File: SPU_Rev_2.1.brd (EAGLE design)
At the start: 127.6 x 101.6 mm, 255 parts, among them Q1 12MHz

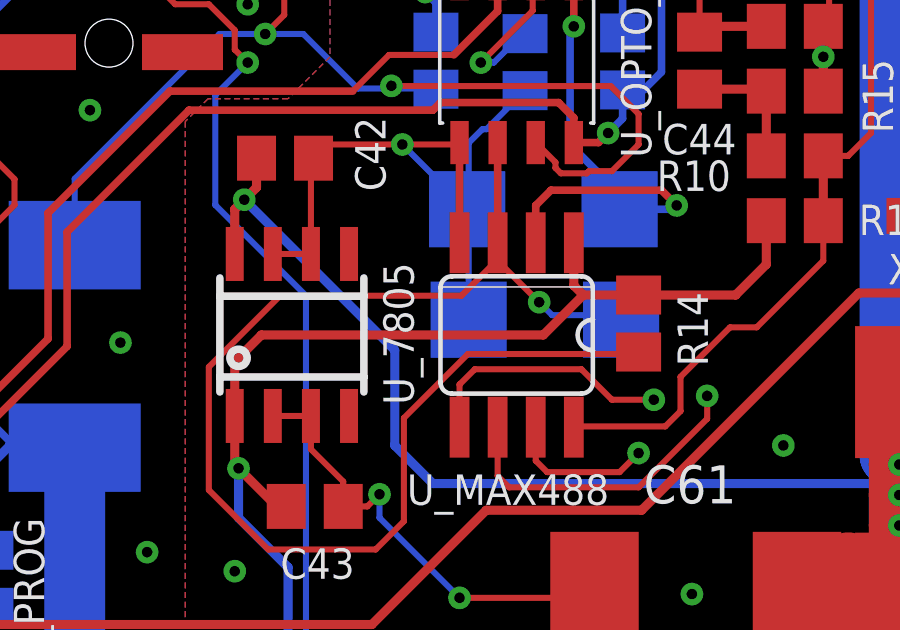
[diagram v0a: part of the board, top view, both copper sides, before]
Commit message: foo
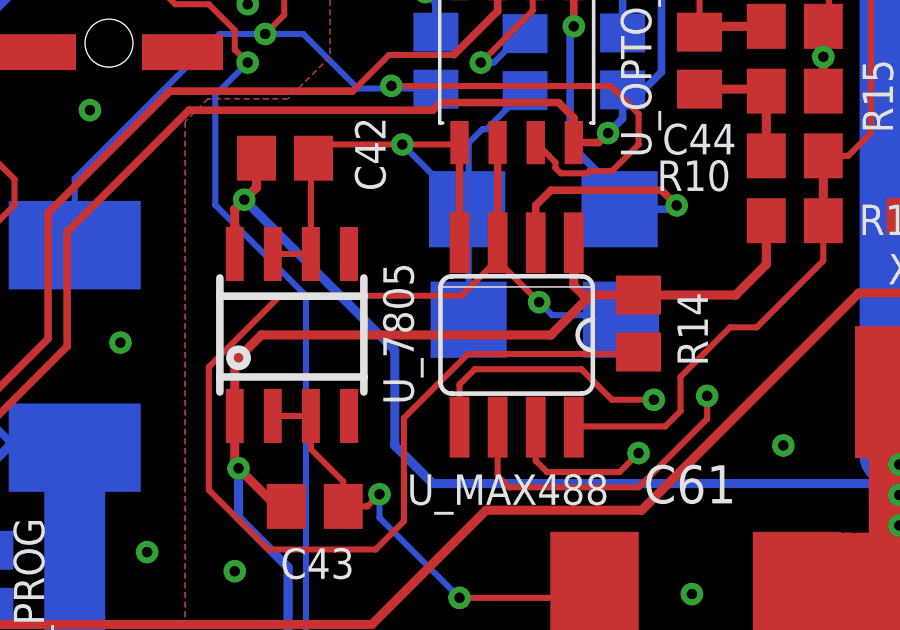
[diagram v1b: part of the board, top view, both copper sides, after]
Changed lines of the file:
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@@
 <drawing>
 <settings>
-<setting alwaysvectorfont="no"/>
+<setting alwaysvectorfont="yes"/>
 <setting verticaltext="up"/>
 </settings>
@@
 <wire x1="15.416" y1="30.783" x2="15.416" y2="31.261" width="0.2032" layer="16"/>
 <wire x1="16.454" y1="34.361" x2="15.367" y2="33.274" width="0.2032" layer="16"/>
-<wire x1="99.568" y1="91.948" x2="101.092" y2="95.123" width="0" layer="19" extent="16-16"/>
-<wire x1="64.4398" y1="61.5696" x2="62.484" y2="61.595" width="0" layer="19" extent="16-16"/>
-<wire x1="40.767" y1="11.176" x2="41.187" y2="9.271" width="0" layer="19" extent="1-1"/>
-<wire x1="71.628" y1="65.532" x2="73.66" y2="66.04" width="0" layer="19" extent="1-1"/>
-<wire x1="12.446" y1="77.597" x2="14.351" y2="78.486" width="0" layer="19" extent="1-1"/>
-<wire x1="38.608" y1="11.176" x2="40.767" y2="11.176" width="0" layer="19" extent="1-1"/>
-<wire x1="91.948" y1="63.881" x2="89.662" y2="63.119" width="0" layer="19" extent="1-1"/>
-<wire x1="90.805" y1="65.532" x2="91.948" y2="63.881" width="0" layer="19" extent="1-1"/>
-<wire x1="91.694" y1="73.787" x2="92.964" y2="71.628" width="0" layer="19" extent="16-16"/>
-<wire x1="97.409" y1="75.565" x2="99.06" y2="77.978" width="0" layer="19" extent="1-1"/>
-<wire x1="86.106" y1="9.525" x2="87.757" y2="7.112" width="0" layer="19" extent="1-1"/>
-<wire x1="67.31" y1="93.98" x2="64.262" y2="94.0054" width="0" layer="19" extent="1-1"/>
-<wire x1="38.735" y1="28.067" x2="39.37" y2="25.019" width="0" layer="19" extent="1-1"/>
-<wire x1="101.346" y1="82.931" x2="99.568" y2="85.598" width="0" layer="19" extent="16-16"/>
-<wire x1="91.694" y1="36.195" x2="91.313" y2="32.893" width="0" layer="19" extent="1-1"/>
-<wire x1="63.881" y1="72.39" x2="62.484" y2="69.215" width="0" layer="19" extent="16-16"/>
-<wire x1="91.186" y1="50.038" x2="89.662" y2="53.286" width="0" layer="19" extent="16-16"/>
-<wire x1="82.169" y1="94.742" x2="78.613" y2="93.8784" width="0" layer="19" extent="1-1"/>
-<wire x1="12.827" y1="26.543" x2="14.732" y2="23.239" width="0" layer="19" extent="1-1"/>
-<wire x1="12.827" y1="6.985" x2="13.208" y2="10.795" width="0" layer="19" extent="1-1"/>
-<wire x1="12.192" y1="84.328" x2="16.013" y2="83.6962" width="0" layer="19" extent="1-1"/>
-<wire x1="32.766" y1="45.212" x2="33.782" y2="49.024" width="0" layer="19" extent="1-1"/>
-<wire x1="26.797" y1="51.562" x2="22.733" y2="51.855" width="0" layer="19" extent="1-1"/>
-<wire x1="59.309" y1="32.512" x2="62.611" y2="30.045" width="0" layer="19" extent="16-16"/>
-<wire x1="102.87" y1="74.168" x2="99.568" y2="71.628" width="0" layer="19" extent="16-16"/>
-<wire x1="105.156" y1="71.755" x2="102.87" y2="74.168" width="0" layer="19" extent="1-1"/>
-<wire x1="103.632" y1="69.088" x2="105.156" y2="71.755" width="0" layer="19" extent="1-1"/>
-<wire x1="25.781" y1="45.339" x2="21.678" y2="46.101" width="0" layer="19" extent="16-16"/>
-<wire x1="40.64" y1="45.339" x2="38.7096" y2="49.149" width="0" layer="19" extent="1-1"/>
-<wire x1="17.272" y1="45.466" x2="19.812" y2="49.024" width="0" layer="19" extent="1-1"/>
-<wire x1="14.516" y1="44.461" x2="17.272" y2="45.466" width="0" layer="19" extent="16-16"/>
-<wire x1="44.577" y1="27.051" x2="42.291" y2="23.239" width="0" layer="19" extent="1-1"/>
-<wire x1="47.752" y1="25.654" x2="44.577" y2="27.051" width="0" layer="19" extent="1-1"/>
-<wire x1="90.17" y1="57.785" x2="89.662" y2="53.286" width="0" layer="19" extent="16-16"/>
-<wire x1="56.769" y1="40.259" x2="61.341" y2="40.767" width="0" layer="19" extent="1-1"/>
-<wire x1="52.832" y1="19.431" x2="48.895" y2="16.891" width="0" layer="19" extent="1-1"/>
-<wire x1="100.965" y1="28.956" x2="100.584" y2="33.909" width="0" layer="19" extent="1-1"/>
-<wire x1="83.693" y1="35.179" x2="78.74" y2="35.56" width="0" layer="19" extent="1-1"/>
-<wire x1="31.496" y1="27.686" x2="29.21" y2="23.239" width="0" layer="19" extent="1-1"/>
-<wire x1="64.262" y1="9.271" x2="69.215" y2="7.205" width="0" layer="19" extent="1-1"/>
-<wire x1="65.532" y1="13.081" x2="64.262" y2="9.271" width="0" layer="19" extent="1-1"/>
-<wire x1="59.817" y1="7.112" x2="64.262" y2="9.271" width="0" layer="19" extent="1-1"/>
-<wire x1="15.416" y1="31.261" x2="12.827" y2="26.543" width="0" layer="19" extent="16-16"/>
-<wire x1="15.748" y1="36.703" x2="17.916" y2="34.361" width="0" layer="19" extent="16-16"/>
-<wire x1="20.701" y1="27.686" x2="22.606" y2="22.567" width="0" layer="19" extent="1-1"/>
-<wire x1="92.075" y1="43.053" x2="86.868" y2="41.214" width="0" layer="19" extent="16-16"/>
-<wire x1="56.515" y1="12.319" x2="57.785" y2="18.034" width="0" layer="19" extent="1-1"/>
-<wire x1="107.188" y1="27.051" x2="100.965" y2="28.956" width="0" layer="19" extent="1-1"/>
-<wire x1="51.054" y1="94.742" x2="50.292" y2="87.576" width="0" layer="19" extent="1-1"/>
-<wire x1="90.043" y1="95.25" x2="82.169" y2="94.742" width="0" layer="19" extent="1-1"/>
-<wire x1="44.069" y1="36.195" x2="35.941" y2="36.068" width="0" layer="19" extent="1-1"/>
-<wire x1="105.664" y1="10.033" x2="96.266" y2="10.734" width="0" layer="19" extent="1-1"/>
-<wire x1="106.553" y1="16.891" x2="105.664" y2="10.033" width="0" layer="19" extent="1-1"/>
 </signal>
 <signal name="28V">
@@
 <wire x1="96.393" y1="44.577" x2="95.123" y2="45.847" width="0.3048" layer="1"/>
 <wire x1="94.996" y1="47.592" x2="94.996" y2="49.403" width="0.3048" layer="1"/>
-<wire x1="106.614" y1="51.623" x2="108.458" y2="51.623" width="0.3048" layer="1"/>
+<wire x1="106.614" y1="51.623" x2="106.868" y2="51.623" width="0.3048" layer="1"/>
+<wire x1="106.868" y1="51.623" x2="108.458" y2="51.623" width="0.3048" layer="1"/>
 <wire x1="94.996" y1="49.403" x2="95.885" y2="50.292" width="0.3048" layer="1"/>
-<wire x1="95.885" y1="50.292" x2="105.283" y2="50.292" width="0.3048" layer="1"/>
-<wire x1="105.283" y1="50.292" x2="106.614" y2="51.623" width="0.3048" layer="1"/>
+<wire x1="95.885" y1="50.292" x2="105.537" y2="50.292" width="0.3048" layer="1"/>
+<wire x1="105.537" y1="50.292" x2="106.868" y2="51.623" width="0.3048" layer="1"/>
 <wire x1="106.299" y1="53.3654" x2="106.299" y2="51.938" width="0.3048" layer="1"/>
 <wire x1="106.299" y1="51.938" x2="106.614" y2="51.623" width="0.3048" layer="1"/>
